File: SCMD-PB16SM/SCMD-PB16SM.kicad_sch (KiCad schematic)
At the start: 30 parts, among them J1 Conn_01x12_Socket, J2 Screw_Terminal_01x02, J3 Screw_Terminal_01x02, M1 SCMD, M10 SCMD, M11 SCMD, M12 SCMD, M2 SCMD, M3 SCMD, M4 SCMD, M5 SCMD, M6 SCMD, M7 SCMD, M8 SCMD, M9 SCMD

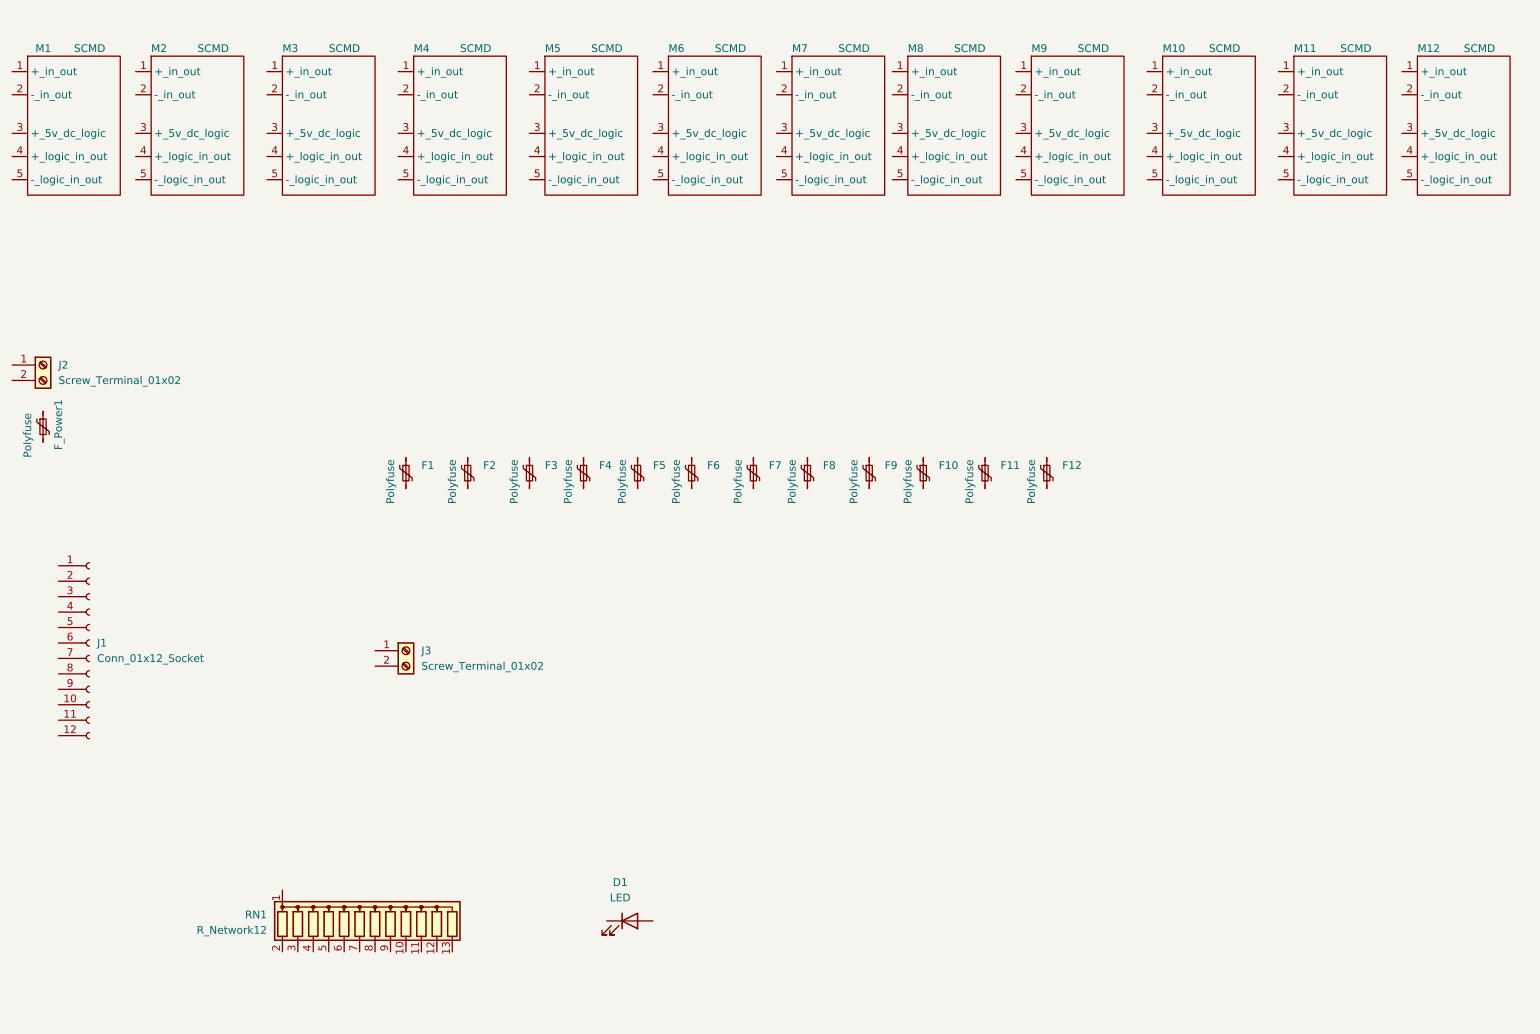
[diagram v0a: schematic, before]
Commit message: Add files via upload
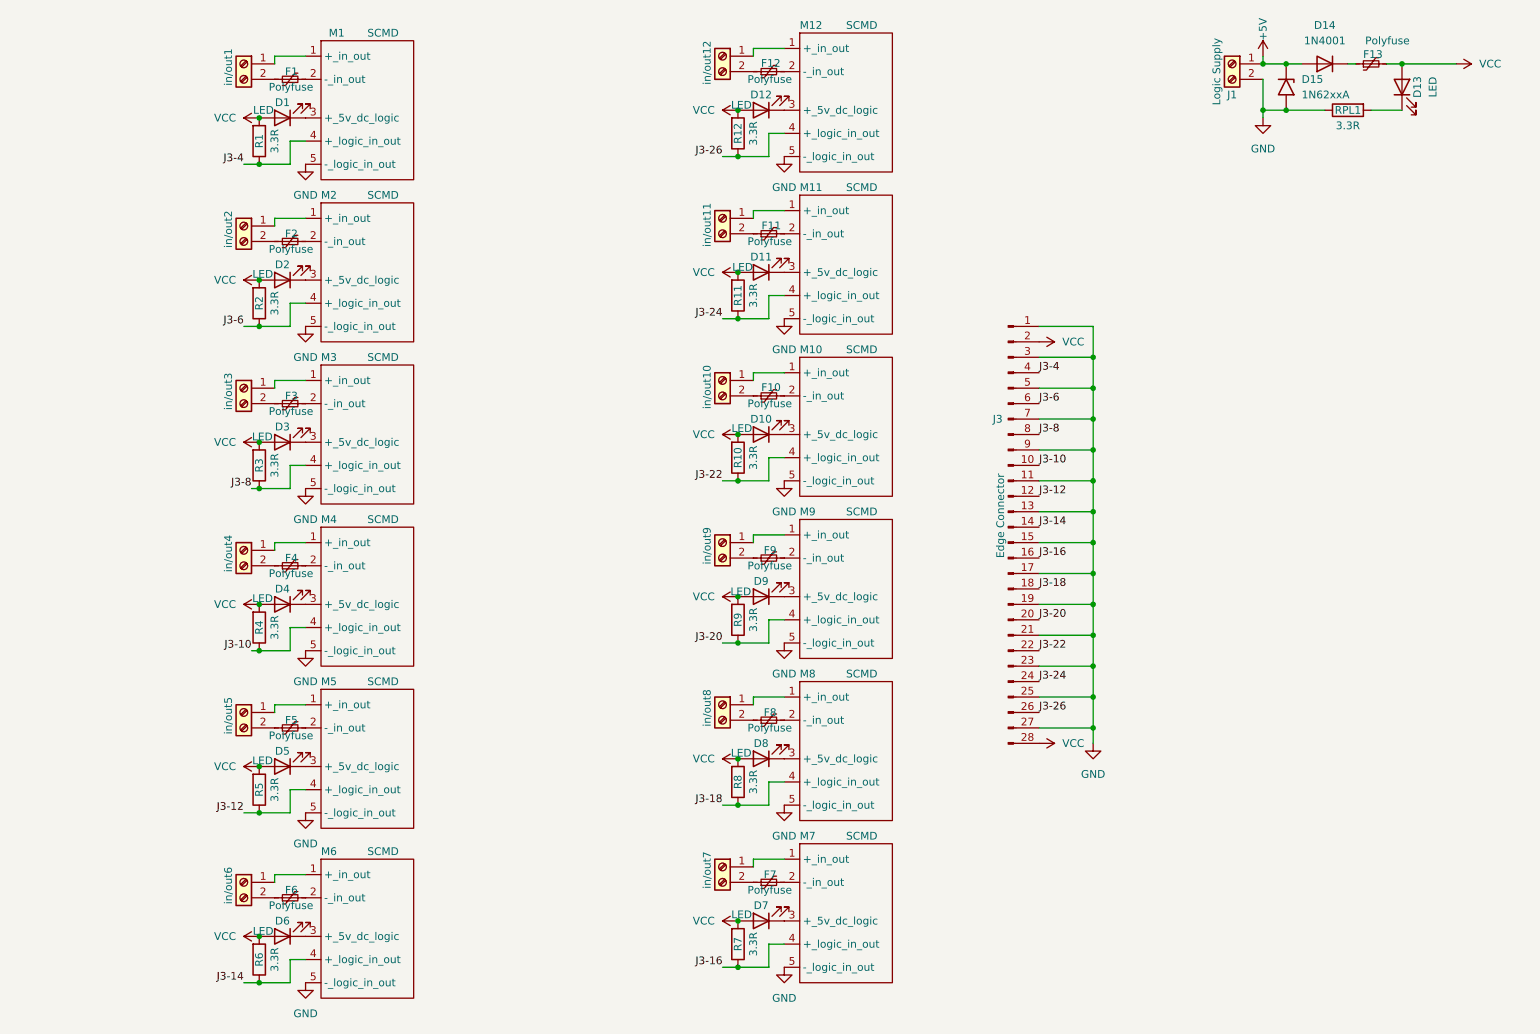
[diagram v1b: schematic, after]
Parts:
- removed J3: Screw_Terminal_01x02, symbol Connector:Screw_Terminal_01x02
- removed RN1: R_Network12, Resistor_THT:R_Array_SIP13, symbol Device:R_Network12
- added D10, D11, D12, D13, D2, D3, D4, D5, D6, D7, D8, D9: LED, LED_THT:LED_D3.0mm_Clear, symbol Device:LED
- added D14: 1N4001, Diode_THT:D_DO-41_SOD81_P10.16mm_Horizontal, symbol Diode:1N4001
- added D15: 1N62xxA, Diode_THT:D_DO-201AE_P15.24mm_Horizontal, symbol Diode:1N62xxA
- added R1, R10, R11, R12, R2, R3, R4, R5, R6, R7, R8, R9, RPL1: 3.3R, Resistor_THT:R_Axial_DIN0204_L3.6mm_D1.6mm_P5.08mm_Horizontal, symbol Device:R
- added in/out1, in/out10, in/out11, in/out12, in/out2, in/out3, in/out4, in/out5, in/out6, in/out7, in/out8, in/out9: Screw_Terminal_01x02, TerminalBlock_Phoenix:TerminalBlock_Phoenix_MPT-0,5-2-2.54_1x02_P2.54mm_Horizontal, symbol Connector:Screw_Terminal_01x02
- D1: footprint (none) -> LED_THT:LED_D3.0mm_Clear
- F1, F10, F11, F12, F2, F3, F4, F5, F6, F7, F8, F9: footprint Fuse:Fuse_BelFuse_0ZRE0100FF_L18.7mm_W5.1mm -> Fuse:Fuse_BelFuse_0ZRE0016FF_L9.9mm_W3.8mm
- F13: renamed from F_Power1; footprint Fuse:Fuse_BelFuse_0ZRE0100FF_L18.7mm_W5.1mm -> Fuse:Fuse_BelFuse_0ZRE0016FF_L9.9mm_W3.8mm
- J1: renamed from J2; value Screw_Terminal_01x02 -> Logic Supply; footprint (none) -> TerminalBlock_Phoenix:TerminalBlock_Phoenix_MPT-0,5-2-2.54_1x02_P2.54mm_Horizontal
- J3: renamed from J1; value Conn_01x12_Socket -> Edge Connector; footprint (none) -> Connector_PinHeader_2.54mm:PinHeader_2x14_P2.54mm_Vertical; symbol Connector:Conn_01x12_Socket -> Connector:Conn_01x28_Pin
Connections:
- net at M3.1 (+_in_out): now also in/out3.1 (Pin_1)
- net at M3.2 (-_in_out): now also F3.2
- net at M3.3 (+_5v_dc_logic): now also D3.1 (K)
- net J3-8: now reaches M3.4 (+_logic_in_out)
- net J3-8: now also J3.8 (Pin_8), R3.1
- net GND: now reaches M3.5 (-_logic_in_out)
- net GND: now also J1.2 (Pin_2), J3.1 (Pin_1), J3.11 (Pin_11), J3.13 (Pin_13), J3.15 (Pin_15), J3.17 (Pin_17), J3.19 (Pin_19), J3.21 (Pin_21), J3.23 (Pin_23), J3.25 (Pin_25), J3.27 (Pin_27), J3.3 (Pin_3), J3.5 (Pin_5), J3.7 (Pin_7), J3.9 (Pin_9), M1.5 (-_logic_in_out), M10.5 (-_logic_in_out), M11.5 (-_logic_in_out), M12.5 (-_logic_in_out), M2.5 (-_logic_in_out), M4.5 (-_logic_in_out), M5.5 (-_logic_in_out), M6.5 (-_logic_in_out), M7.5 (-_logic_in_out), M8.5 (-_logic_in_out), M9.5 (-_logic_in_out), D15.2 (A2), RPL1.1
- net at F10.1: now also in/out10.2 (Pin_2)
- net at F10.2: now also M10.2 (-_in_out)
- net at F13.1: now also D14.1 (K)
- net VCC: now reaches F13.2
- net VCC: now also D1.2 (A), J3.2 (Pin_2), J3.28 (Pin_28), D10.2 (A), D11.2 (A), D12.2 (A), D13.2 (A), D2.2 (A), D3.2 (A), D4.2 (A), D5.2 (A), D6.2 (A), D7.2 (A), D8.2 (A), D9.2 (A), R1.2, R10.2, R11.2, R12.2, R2.2, R3.2, R4.2, R5.2, R6.2, R7.2, R8.2, R9.2
- net at M2.1 (+_in_out): now also in/out2.1 (Pin_1)
- net at M2.2 (-_in_out): now also F2.2
- net at M2.3 (+_5v_dc_logic): now also D2.1 (K)
- net J3-6: now reaches M2.4 (+_logic_in_out)
- net J3-6: now also J3.6 (Pin_6), R2.1
- net at M9.1 (+_in_out): now also in/out9.1 (Pin_1)
- net at M9.2 (-_in_out): now also F9.2
- net at M9.3 (+_5v_dc_logic): now also D9.1 (K)
- net J3-20: now reaches M9.4 (+_logic_in_out)
- net J3-20: now also J3.20 (Pin_20), R9.1
- net at M6.1 (+_in_out): now also in/out6.1 (Pin_1)
- net at M6.2 (-_in_out): now also F6.2
- net at M6.3 (+_5v_dc_logic): now also D6.1 (K)
- net J3-14: now reaches M6.4 (+_logic_in_out)
- net J3-14: now also J3.14 (Pin_14), R6.1
- net at M11.1 (+_in_out): now also in/out11.1 (Pin_1)
- net at M11.2 (-_in_out): now also F11.2
- net at M11.3 (+_5v_dc_logic): now also D11.1 (K)
- net J3-24: now reaches M11.4 (+_logic_in_out)
- net J3-24: now also J3.24 (Pin_24), R11.1
- net at M1.1 (+_in_out): now also in/out1.1 (Pin_1)
- net at M1.2 (-_in_out): now also F1.2
- net at M1.3 (+_5v_dc_logic): now also D1.1 (K)
- net J3-4: now reaches M1.4 (+_logic_in_out)
- net J3-4: now also J3.4 (Pin_4), R1.1
- net at F1.1: now also in/out1.2 (Pin_2)
- net at F3.1: now also in/out3.2 (Pin_2)
- net at F12.1: now also in/out12.2 (Pin_2)
- net at F12.2: now also M12.2 (-_in_out)
- net at M12.1 (+_in_out): now also in/out12.1 (Pin_1)
- net at M12.3 (+_5v_dc_logic): now also D12.1 (K)
- net J3-26: now reaches M12.4 (+_logic_in_out)
- net J3-26: now also J3.26 (Pin_26), R12.1
- net at M7.1 (+_in_out): now also in/out7.1 (Pin_1)
- net at M7.2 (-_in_out): now also F7.2
- net at M7.3 (+_5v_dc_logic): now also D7.1 (K)
- net J3-16: now reaches M7.4 (+_logic_in_out)
- net J3-16: now also J3.16 (Pin_16), R7.1
- net at M10.1 (+_in_out): now also in/out10.1 (Pin_1)
- net at M10.3 (+_5v_dc_logic): now also D10.1 (K)
- net J3-22: now reaches M10.4 (+_logic_in_out)
- net J3-22: now also J3.22 (Pin_22), R10.1
- net at F8.1: now also in/out8.2 (Pin_2)
- net at F8.2: now also M8.2 (-_in_out)
- net at M4.1 (+_in_out): now also in/out4.1 (Pin_1)
- net at M4.2 (-_in_out): now also F4.2
- net at M4.3 (+_5v_dc_logic): now also D4.1 (K)
- net J3-10: now reaches M4.4 (+_logic_in_out)
- net J3-10: now also J3.10 (Pin_10), R4.1
- net at M8.1 (+_in_out): now also in/out8.1 (Pin_1)
- net at M8.3 (+_5v_dc_logic): now also D8.1 (K)
- net J3-18: now reaches M8.4 (+_logic_in_out)
- net J3-18: now also J3.18 (Pin_18), R8.1
- net at F7.1: now also in/out7.2 (Pin_2)
- net at F4.1: now also in/out4.2 (Pin_2)
- net J3-12: now reaches J3.12 (Pin_12)
- net J3-12: now also M5.4 (+_logic_in_out), R5.1
- net at F9.1: now also in/out9.2 (Pin_2)
- net at F11.1: now also in/out11.2 (Pin_2)
- net at M5.1 (+_in_out): now also in/out5.1 (Pin_1)
- net at M5.2 (-_in_out): now also F5.2
- net at M5.3 (+_5v_dc_logic): now also D5.1 (K)
- net at F5.1: now also in/out5.2 (Pin_2)
- net at F6.1: now also in/out6.2 (Pin_2)
- net +5V: now reaches J1.1 (Pin_1)
- net +5V: now also D14.2 (A), D15.1 (A1)
- net at F2.1: now also in/out2.2 (Pin_2)
- new net: D13.1 (K), RPL1.2
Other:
- moved on the sheet: D1, F1, F10, F11, F12, F13, F2, F3, F4, F5, F6, F7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
